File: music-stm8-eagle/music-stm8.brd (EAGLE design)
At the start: 76.2 x 48.9 mm, 37 parts, among them IC1 STM8S105K6T, IC2 REG1117, J1 CON-SD-MMC-1, Q1 24.576mHz, Q2 8mHz, X1 SJ-3524-SMT, X2 MINI-USB-32005-301

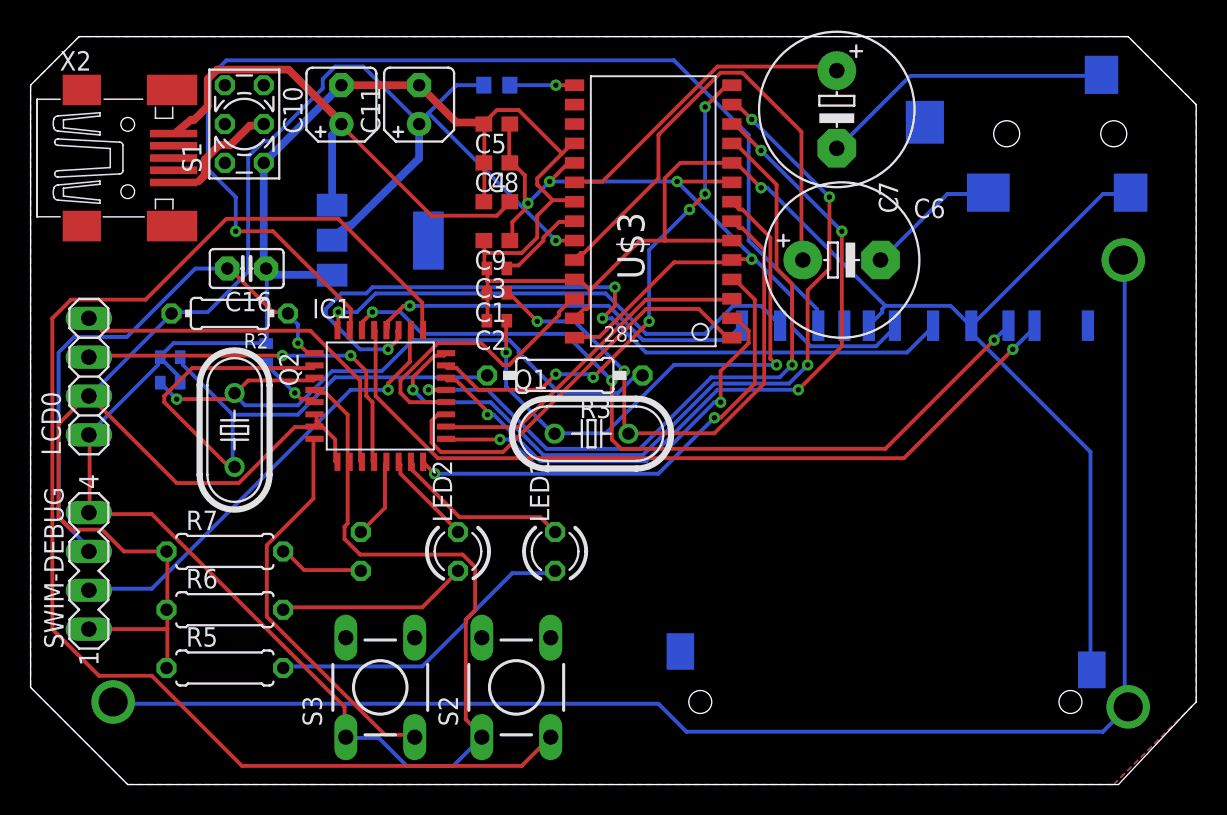
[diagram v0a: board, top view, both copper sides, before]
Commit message: mistakes regarding pcb
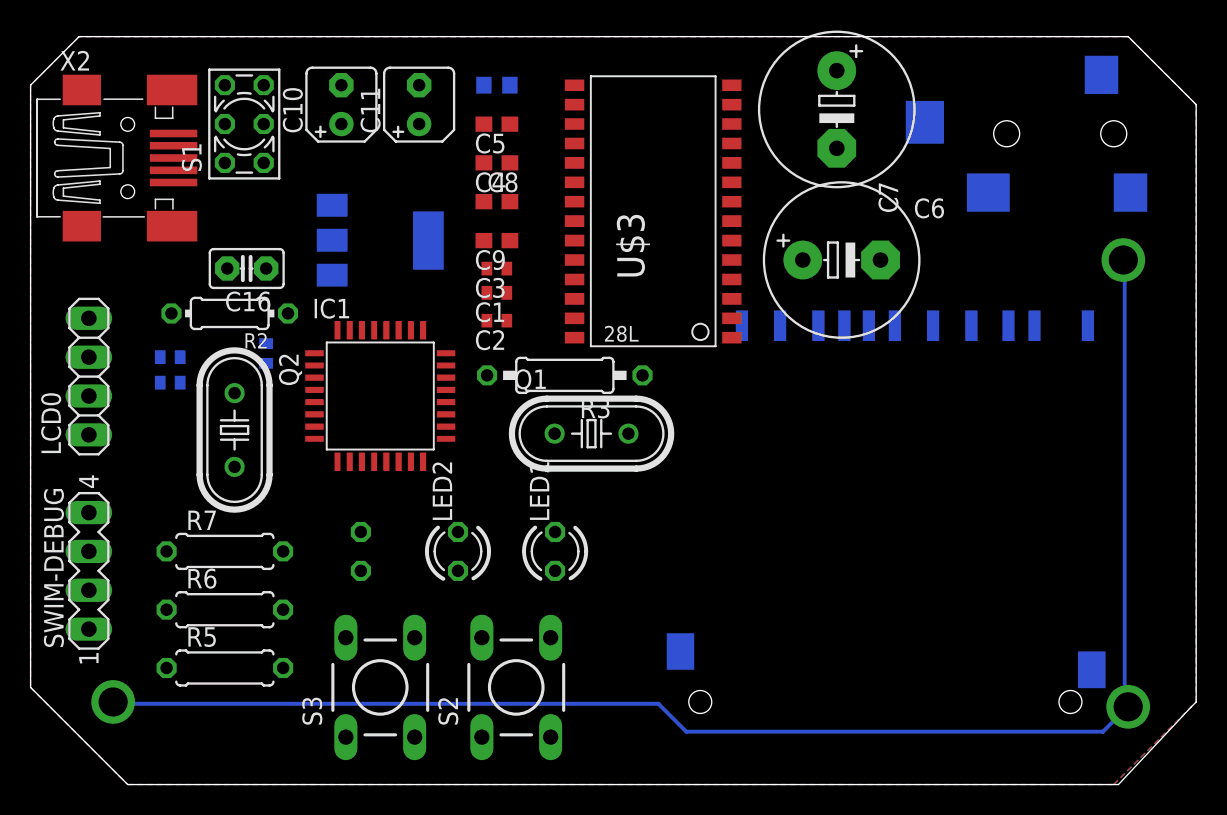
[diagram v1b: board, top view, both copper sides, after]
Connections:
- net N$18: no longer R3.2
- net N$19: no longer R3.1
- net N$2: now also R3.2
- net N$6: now also R3.1
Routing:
- net GND: track 244.2 -> 0.00 mm, vias 1 -> 0
- net VDD: track 177.7 -> 0.00 mm, vias 5 -> 0
- net N$36: track 88.3 -> 0.00 mm
- net N$20: track 74.0 -> 0.00 mm, vias 1 -> 0
- net N$5: track 54.1 -> 0.00 mm, vias 4 -> 0
- net N$26: track 52.8 -> 0.00 mm, vias 1 -> 0
- net N$25: track 52.3 -> 0.00 mm, vias 3 -> 0
- net N$22: track 52.1 -> 0.00 mm, vias 3 -> 0
- net N$7: track 49.1 -> 0.00 mm, vias 4 -> 0
- net N$8: track 45.2 -> 0.00 mm, vias 2 -> 0
- net N$18: track 43.8 -> 0.00 mm
- net N$19: track 42.0 -> 0.00 mm, vias 1 -> 0
- net N$6: track 37.1 -> 0.00 mm, vias 2 -> 0
- net N$17: track 35.9 -> 0.00 mm, vias 1 -> 0
- net N$2: track 35.9 -> 0.00 mm, vias 2 -> 0
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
